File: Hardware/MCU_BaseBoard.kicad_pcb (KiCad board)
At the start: 2 copper layers, 156 parts, among them IC1 L293D, IC2 LM1117, J1 USB_2, K1 RELAYPTH, K2 RELAYPTH, K3 I2C, K4 CONN_3, P1 CONN_01X04, P10 CONN_1, P11 CONN_4, P12 CONN_8, P13 CONN_1, P14 CONN_01X10, P15 CONN_01X10, P16 CONN_01X10, P17 CONN_01X10, P18 CONN_01X10, P19 CONN_01X10, P2 CONN_01X10, P20 CONN_01X10, P21 CONN_01X01, P22 CONN_01X03, P23 CONN_01X01, P24 CONN_01X01, P25 CONN_01X04, P26 CONN_01X04, P27 CONN_01X04, P28 CONN_01X05, P29 CONN_01X04, P3 CONN_01X04, P4 CONN_01X04, P5 CONN_01X04, P6 CONN_1, P7 CONN_1, P8 CONN_1, P9 CONN_1, Q1 BC547, Q2 BC547, Q3 BC547, Q4 BC547, Q5 BC547, Q6 BC547, Q7 BC547, SW1 INT1, SW10 5, SW11 6, SW12 7, SW13 8, SW14 1, SW15 2, SW16 3, SW17 4, SW18 INT0, SW19 INT1, SW2 C, SW20 SPST, SW21 INT1, SW3 D, SW4 E, SW5 F, SW6 9, SW7 0, SW8 A, SW9 B, U1 7805, U2 24C16, U3 DS1307, U4 BATTERY, U6 CONN_15, U7 LCD-jhd12864e-xl, U8 CP2102, X1 CRYSTAL

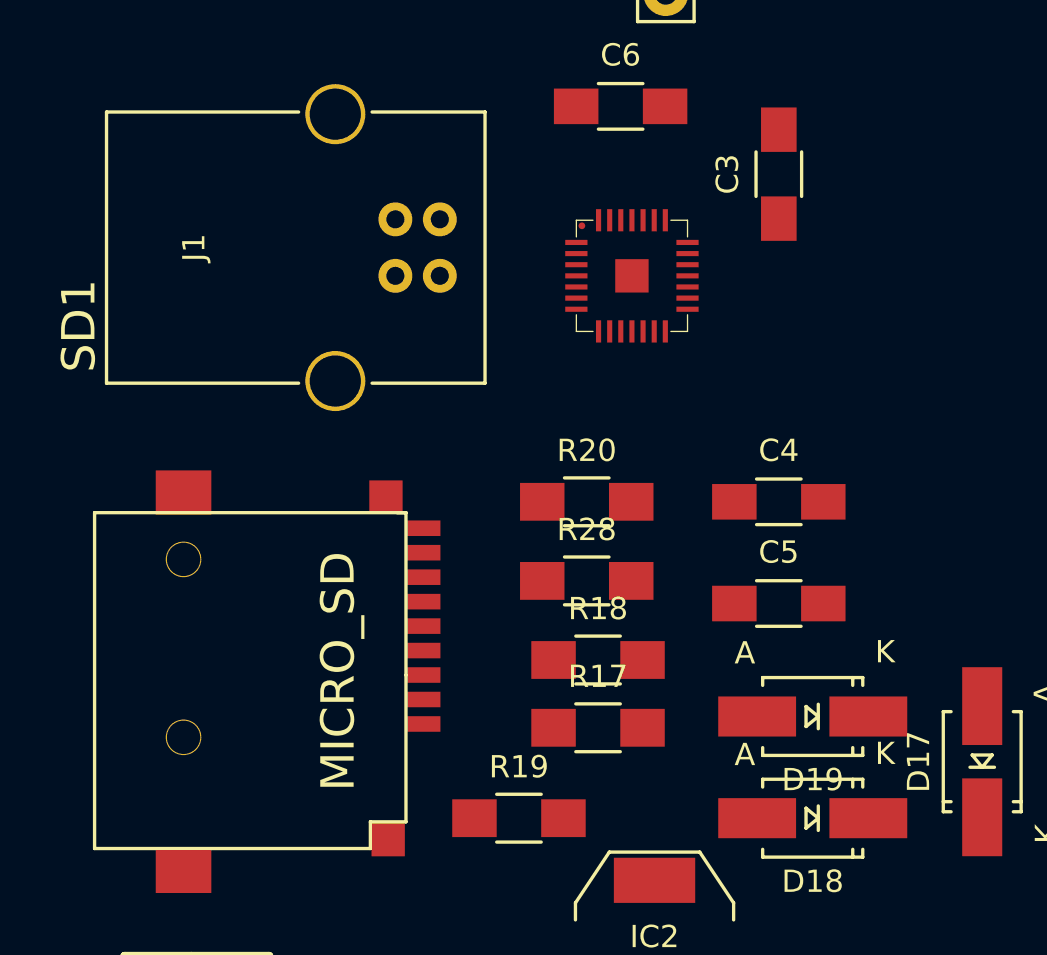
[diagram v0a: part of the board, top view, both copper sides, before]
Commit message: test
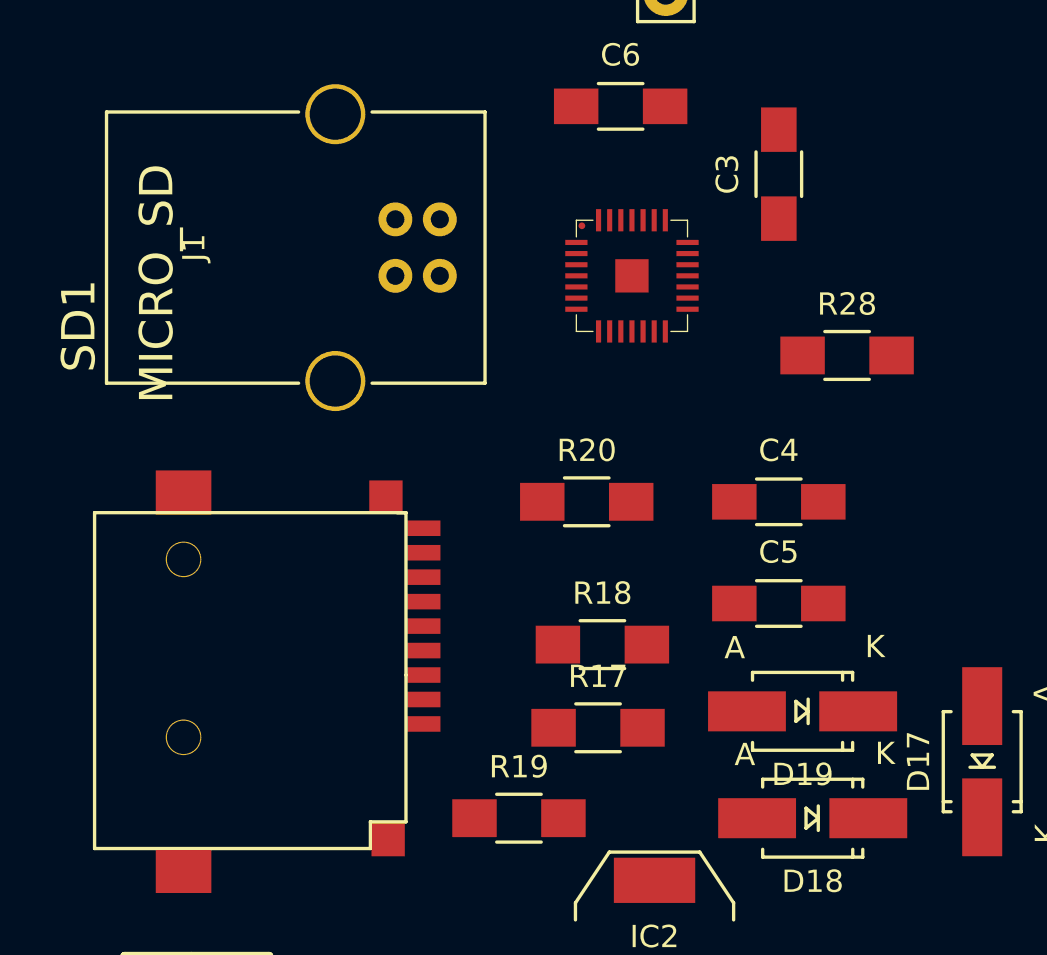
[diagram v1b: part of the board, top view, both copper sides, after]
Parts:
- moved R28 15.5 mm to (94.0, 62.0)
- moved R18 0.72 mm to (83.0, 75.0)
- moved D19 0.51 mm to (92.0, 78.0)
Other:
- board text removed: "1. Make legend such that it shows which LCD should be placed where 2. Mounting holes for LCDs"
- board text removed: "USE smd regulartor and bridge, no need for head sink."
- board text removed: "can this be horizontal?"
- board text removed: "check segment legend"
- board text removed: "make single 40 pin footprint"
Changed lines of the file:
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@@
     (area 31.285716 -120 247.493952 191.529)
     (thickness 1.6)
-    (drawings 36)
+    (drawings 27)
     (tracks 0)
     (zones 0)
@@
   )
   (module Diodes_SMD:Diode-SMA_Handsoldering (layer F.Cu)
-    (at 92.456 78.232 180)
+    (at 92 78 180)
     (descr "Diode SMA Handsoldering")
     (tags "Diode SMA Handsoldering")
@@
   )
   (module Resistors_SMD:R_1206_HandSoldering (layer F.Cu)
-    (at 82.804 75.692)
+    (at 83 75)
     (descr "Resistor SMD 1206, hand soldering")
     (tags "resistor 1206")
@@
   )
   (module Resistors_SMD:R_1206_HandSoldering (layer F.Cu)
-    (at 82.296 72.136)
+    (at 94 62)
     (descr "Resistor SMD 1206, hand soldering")
     (tags "resistor 1206")
@@
       (effects (font (size 1.5 1.5) (thickness 0.15)))
     )
-    (fp_text value MICRO_SD (at 2.032 3.048 270) (layer F.SilkS)
+    (fp_text value MICRO_SD (at -15.4 11.2 270) (layer F.SilkS)
       (effects (font (size 1.5 1.5) (thickness 0.15)))
     )
@@
     )
   )
-  (gr_text "can this be horizontal?\n" (at 175.26 30.48) (layer Dwgs.User)
-    (effects (font (size 1.5 1.5) (thickness 0.3)))
-  )
-  (gr_line (start 175.26 41.91) (end 177.8 39.37) (angle 90) (layer Dwgs.User) (width 0.2))
-  (gr_line (start 172.72 39.37) (end 175.26 41.91) (angle 90) (layer Dwgs.User) (width 0.2))
-  (gr_line (start 175.26 31.75) (end 173.99 31.75) (angle 90) (layer Dwgs.User) (width 0.2))
-  (gr_line (start 175.26 41.91) (end 175.26 31.75) (angle 90) (layer Dwgs.User) (width 0.2))
-  (gr_text "check segment legend" (at 213.36 53.34) (layer Dwgs.User)
-    (effects (font (size 1.5 1.5) (thickness 0.3)))
-  )
-  (gr_text "1. Make legend such that it shows \nwhich LCD should be placed where\n\n2. Mounting holes for LCDs" (at 127 59.69) (layer Dwgs.User)
-    (effects (font (size 1.5 1.5) (thickness 0.3)))
-  )
-  (gr_text "USE smd regulartor and bridge, no need for head sink. " (at 67.31 118.11) (layer Dwgs.User)
-    (effects (font (size 1.5 1.5) (thickness 0.3)))
-  )
-  (gr_text "make single 40 pin footprint" (at 129.54 140.97) (layer Cmts.User)
-    (effects (font (size 1.5 1.5) (thickness 0.3)))
-  )
   (gr_line (start 191 107) (end 191 108) (angle 90) (layer F.Fab) (width 0.2))

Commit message: added new files
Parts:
- removed C6: 0.1uf, Capacitors_SMD:C_1206_HandSoldering
- removed J1: USB_2, Connect:USB_B
- removed P18, P19, P20: CONN_01X10, Pin_Headers:Pin_Header_Straight_1x10
- removed P21, P23, P24: CONN_01X01, Pin_Headers:Pin_Header_Straight_1x01
- removed R11, R12: 10k, Resistors_SMD:R_1206_HandSoldering
- removed SW1, SW21: INT1, sw:SW_PUSH_SMALL_2pin_3D_xl
- removed U6: CONN_15, Pin_Headers:Pin_Header_Straight_1x15
- removed U8: CP2102, sw:cp2102_xl2
- added P30: CONN_01X07, Pin_Headers:Pin_Header_Straight_1x07, F.Cu at (76.0, 33.0)
- added P31: CONN_01X08, Pin_Headers:Pin_Header_Straight_1x08, F.Cu at (73.2, 99.6)
- added P32: CONN_01X05, Pin_Headers:Pin_Header_Straight_1x05, F.Cu at (96.0, 99.6)
- added U5: 40PIN_Breakout, sw:40pin_breakout, F.Cu at (168.4, 108.5)
- AFF1, AFF2, AFF3, AFF4: footprint Displays_7-Segment:LTS-69xx -> Displays_7-Segment:7SegmentLED_LTS6760_LTS6780
- C4, C5: moved to B.Cu
- D1: footprint sw:W005M_XL -> sw:bridge_smd_xl
- LCD1: footprint Pin_Headers:Pin_Header_Straight_1x16 -> Display:WC1602A
- P1: value CONN_01X04 -> CONN_01X02; footprint Pin_Headers:Pin_Header_Straight_1x04 -> Pin_Headers:Pin_Header_Straight_1x02
- P14, P2: value CONN_01X10 -> CONN_01X20; footprint Pin_Headers:Pin_Header_Straight_1x10 -> Pin_Headers:Pin_Header_Straight_1x20
- P15: value CONN_01X10 -> CONN_01X03; footprint Pin_Headers:Pin_Header_Straight_1x10 -> Pin_Headers:Pin_Header_Straight_1x03
- P16: value CONN_01X10 -> CONN_01X06; footprint Pin_Headers:Pin_Header_Straight_1x10 -> Pin_Headers:Pin_Header_Straight_1x06
- P17: value CONN_01X10 -> CONN_01X04; footprint Pin_Headers:Pin_Header_Straight_1x10 -> Pin_Headers:Pin_Header_Straight_1x04
- X1: value CRYSTAL -> CRYSTAL_SMD; footprint Pin_Headers:Pin_Header_Straight_1x02 -> sw:RTC_Crystal
- moved P9 288.0 mm to (46.0, 146.0)
- moved P29 143.5 mm to (206.8, 146.9)
- moved P6 121.2 mm to (132.9, 87.5)
- moved JP9 117.4 mm to (217.0, 68.0), turned to 90 degrees
- moved P14 116.9 mm to (193.8, 85.6)
- moved JP8 107.1 mm to (217.0, 79.0), turned to 90 degrees
- moved IC1 95.8 mm to (190.0, 73.4), turned to 0 degrees
- moved P16 95.1 mm to (99.1, 63.2), turned to 90 degrees
- moved SW14 91.8 mm to (104.3, 144.7)
- moved SW10 84.7 mm to (104.3, 135.8)
- moved SW15 84.3 mm to (113.8, 144.7)
- moved JP10 80.4 mm to (133.1, 108.2), turned to 90 degrees
- moved JP6 80.1 mm to (208.0, 70.0), turned to 0 degrees
- moved SW6 79.1 mm to (104.3, 126.9)
- moved SW11 78.6 mm to (113.8, 135.8)
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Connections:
- P14 pad 1: Net-(P14-Pad1) -> +5V
- P14 pad 2: RST -> GND
- P15 pad 1: RX -> /ADC/IN2
- P15 pad 2: TX -> /ADC/POT
- P15 pad 3: Net-(P15-Pad3) -> /ADC/TS
- P16 pad 1: Net-(P14-Pad1) -> 3.3V
- P16 pad 2: RST -> GND
- P16 pad 3: Net-(P14-Pad3) -> Net-(P16-Pad3)
- P16 pad 4: Net-(P14-Pad4) -> Net-(P16-Pad4)
- P16 pad 5: Net-(P14-Pad5) -> Net-(P16-Pad5)
- P16 pad 6: Net-(P14-Pad6) -> Net-(P16-Pad6)
- P17 pad 1: +5V -> Net-(P16-Pad3)
- P17 pad 2: GND -> Net-(P16-Pad4)
- P17 pad 3: Net-(P17-Pad3) -> Net-(P16-Pad5)
- P17 pad 4: Net-(P17-Pad4) -> Net-(P16-Pad6)
- P2 pad 10: Net-(P15-Pad10) -> Net-(P2-Pad10)
- P2 pad 3: Net-(P15-Pad3) -> Net-(P2-Pad3)
- P2 pad 4: Net-(P15-Pad4) -> Net-(P2-Pad4)
- P2 pad 5: Net-(P15-Pad5) -> Net-(P2-Pad5)
- P2 pad 6: Net-(P15-Pad6) -> Net-(P2-Pad6)
- P2 pad 7: Net-(P15-Pad7) -> Net-(P2-Pad7)
- P2 pad 8: Net-(P15-Pad8) -> Net-(P2-Pad8)
- P2 pad 9: Net-(P15-Pad9) -> Net-(P2-Pad9)
- RV1 pad 2: Net-(P21-Pad1) -> /ADC/TS
- RV2 pad 2: Net-(P23-Pad1) -> /ADC/POT
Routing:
- net GND: track 0.00 -> 1043.5 mm, vias 0 -> 11
- net +5V: track 0.00 -> 778.7 mm, vias 0 -> 7
- net 3.3V: track 0.00 -> 387.6 mm, vias 0 -> 10
- net 9V/12V: track 0.00 -> 327.8 mm
- net RX: track 0.00 -> 230.0 mm, vias 0 -> 1
- net TX: track 0.00 -> 224.7 mm, vias 0 -> 1
- net /ADC/SSEL: track 0.00 -> 159.2 mm, vias 0 -> 3
- net VO: track 0.00 -> 138.6 mm, vias 0 -> 2
- net /ADC/SCK: track 0.00 -> 138.2 mm, vias 0 -> 3
- net /ADC/MOSI: track 0.00 -> 135.1 mm, vias 0 -> 3
- net /ADC/MISO: track 0.00 -> 114.0 mm, vias 0 -> 3
- net RS: track 0.00 -> 100.9 mm, vias 0 -> 1
- net Net-(JP10-Pad1): track 0.00 -> 99.4 mm, vias 0 -> 1
- net DATA3: track 0.00 -> 98.5 mm, vias 0 -> 2
- net E: track 0.00 -> 96.9 mm, vias 0 -> 2
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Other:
- board outline added: 180 x 125 mm
- board text added: "+5V"
- board text added: "16X2 LCD"
- board text added: "3.3V"
- board text added: "5V"
- board text added: "9/12V"
- board text added: "ADC_REF"
- board text added: "BUZZER"
- board text added: "C"
- board text added: "C1"
- board text added: "C2"
- board text added: "C3"
- board text added: "C4"
- board text added: "CD"
- board text added: "CS"
- board text added: "CS1"
- board text added: "CS2"
- board text added: "D0"
- board text added: "D1"
- board text added: "D2"
- board text added: "D3"
- board text added: "D4"
- board text added: "D5"
- board text added: "D6"
- board text added: "D7"
- board text added: "DTR"
- board text added: "E"
- board text added: "GLCD"
- board text added: "GND"
- board text added: "INTR_S1"
- board text added: "INTR_S2"
- board text added: "LDR"
- board text added: "M1a"
- board text added: "M1b"
- board text added: "M2a"
- board text added: "M2b"
- board text added: "MISO"
- board text added: "MOSI"
- board text added: "MOTOR1"
- board text added: "MOTOR2"
- board text added: "NC"
- board text added: "NO"
- board text added: "OUT"
- board text added: "POT"
- board text added: "R1"
- board text added: "R2"
- board text added: "R3"
- board text added: "R4"
- board text added: "RL1"
- board text added: "RL2"
- board text added: "RS"
- board text added: "RX"
- board text added: "S1"
- board text added: "S2"
- board text added: "S3"
- board text added: "S4"
- board text added: "SCK"
- board text added: "SCL"
- board text added: "SDA"
- board text added: "SSEL"
- board text added: "TEMP"
- board text added: "TX"
- board text added: "W"
- board text added: "a"
- board text added: "b"
- board text added: "c"
- board text added: "d"
- board text added: "e"
- board text added: "f"
- board text added: "g"
- board text added: "h"
